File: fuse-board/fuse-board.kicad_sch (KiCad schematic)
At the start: 27 parts, among them J1 FTSH-107-01-F-DV-K-P-TR, J2 74651173R, J3 74651173R, J4 ATM15-12PA-BM04, J5 1053141106, SW1 Y97KT23B5NAFP, U1 STM32G491KCUx, U2 AP63205WU, U3 MIC5504-3.3YM5, Y1 ECS-240-8-37B-CKY-TR

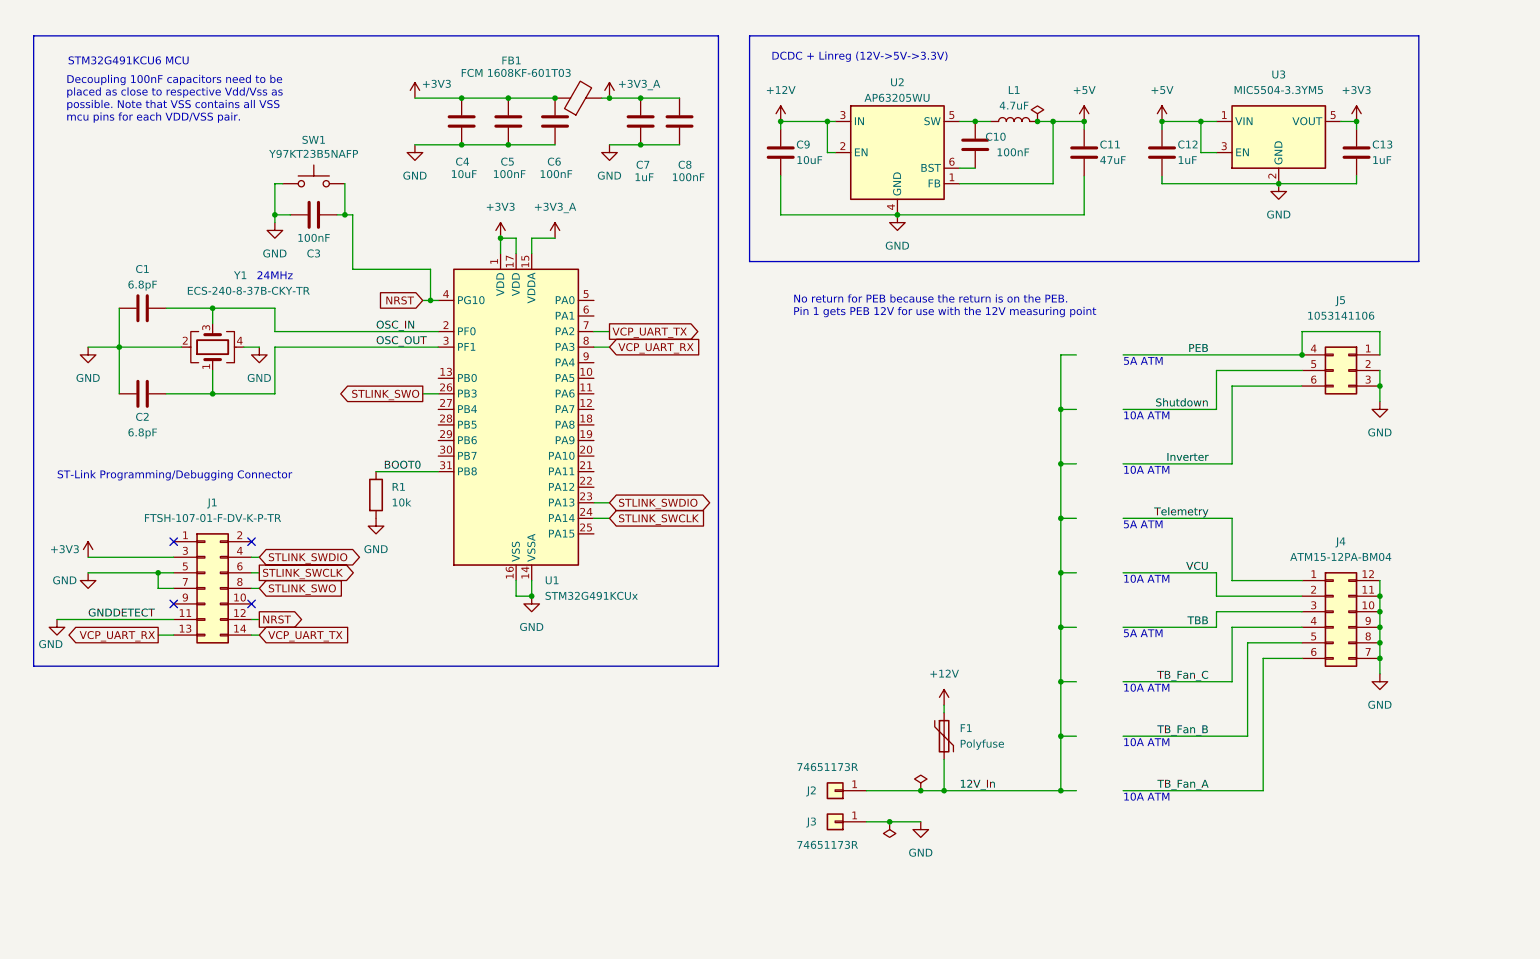
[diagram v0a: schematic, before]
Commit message: add efuses and sheets
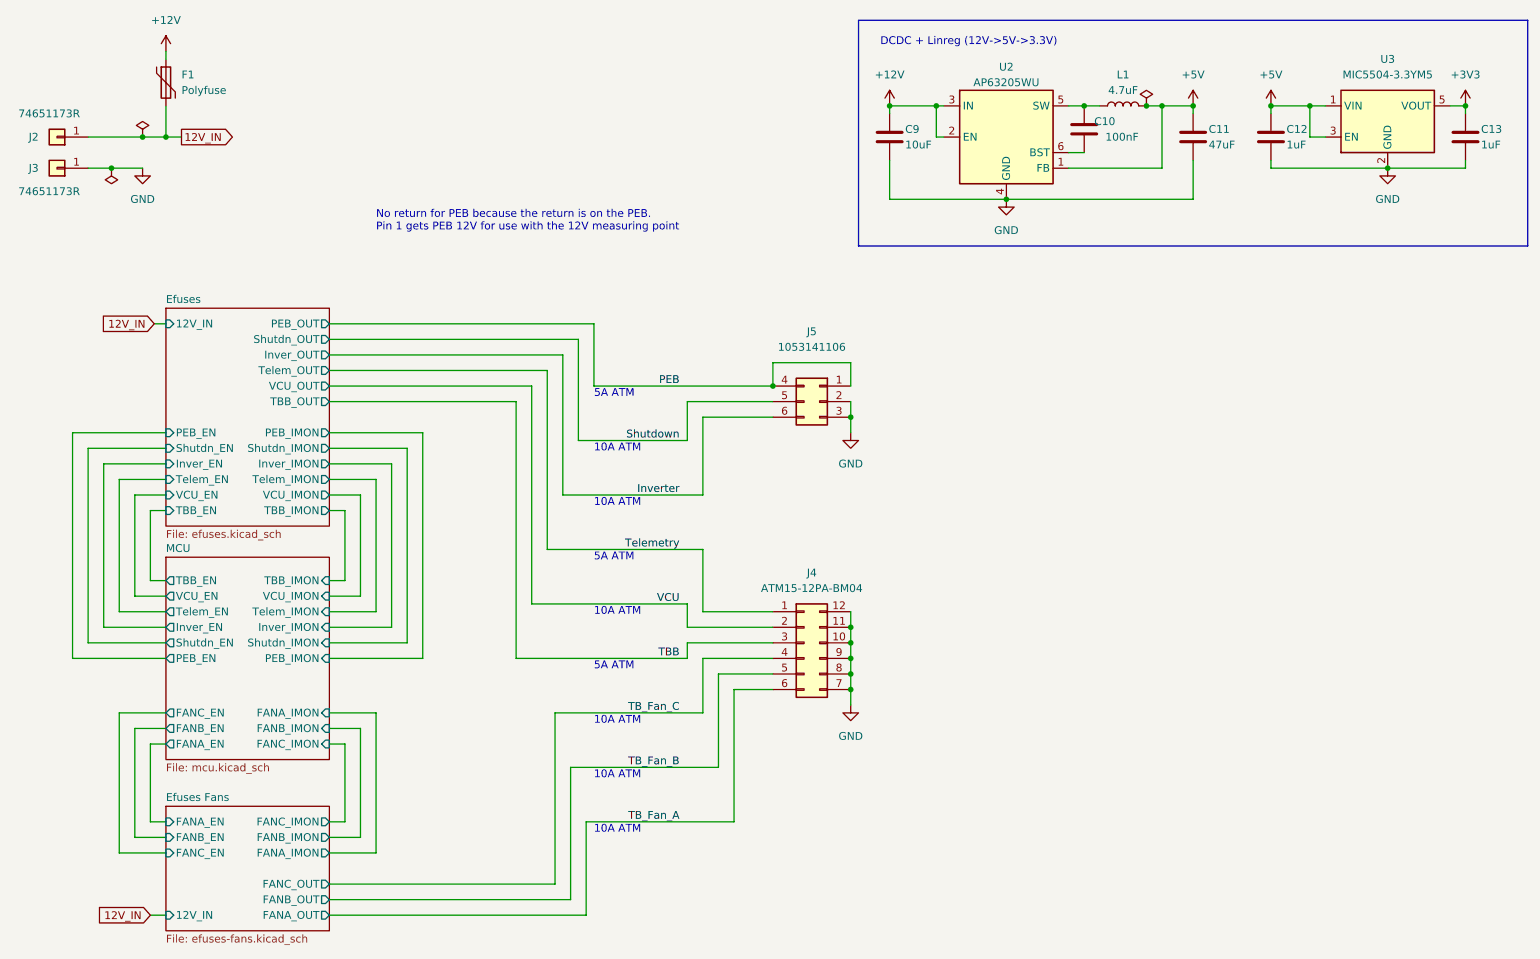
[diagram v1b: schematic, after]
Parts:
- removed C1, C2: 6.8pF, Capacitor_SMD:C_0603_1608Metric_Pad1.08x0.95mm_HandSolder, symbol Device:C
- removed C3, C5, C6, C8: 100nF, Capacitor_SMD:C_0603_1608Metric_Pad1.08x0.95mm_HandSolder, symbol Device:C
- removed C4: 10uF, Capacitor_SMD:C_0603_1608Metric_Pad1.08x0.95mm_HandSolder, symbol Device:C
- removed C7: 1uF, Capacitor_SMD:C_0603_1608Metric_Pad1.08x0.95mm_HandSolder, symbol Device:C
- removed FB1: FCM 1608KF-601T03, Inductor_SMD:L_0603_1608Metric_Pad1.05x0.95mm_HandSolder, symbol Device:FerriteBead
- removed J1: FTSH-107-01-F-DV-K-P-TR, Connector_PinHeader_1.27mm:PinHeader_2x07_P1.27mm_Vertical_SMD, symbol Connector_Generic:Conn_02x07_Odd_Even
- removed R1: 10k, Resistor_SMD:R_0603_1608Metric_Pad0.98x0.95mm_HandSolder, symbol Device:R
- removed SW1: Y97KT23B5NAFP, Button_Switch_SMD:SW_SPST_PTS647_Sx38, symbol Switch:SW_Push
- removed U1: STM32G491KCUx, Package_DFN_QFN:QFN-32-1EP_5x5mm_P0.5mm_EP3.45x3.45mm, symbol MCU_ST_STM32G4:STM32G491KCUx
- removed Y1: ECS-240-8-37B-CKY-TR, Crystal:Crystal_SMD_2016-4Pin_2.0x1.6mm, symbol Device:Crystal_GND24
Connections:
- net 12V_In renamed 12V_IN
- no-connect marks 4 -> 0
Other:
- added sheet Efuses (efuses.kicad_sch)
- added sheet Efuses Fans (efuses-fans.kicad_sch)
- added sheet MCU (mcu.kicad_sch)
- note removed: "24MHz"
- note removed: "Decoupling 100nF capacitors need to be placed as close to respective Vdd/Vss as possible. Note that VSS contains all VSS mcu pins for each VDD/VSS pair."
- note removed: "ST-Link Programming/Debugging Connector"
- note removed: "STM32G491KCU6 MCU"
- moved on the sheet: C10, C11, C12, C13, C9, L1, U2, U3
